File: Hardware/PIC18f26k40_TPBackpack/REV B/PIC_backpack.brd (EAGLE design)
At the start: 45 x 57.5 mm, 61 parts, among them IC1 PIC18F2480-I/ML, T1 BT138-V, T2 BT138-V, U4 W5500, Y2 CRYSTAL-GROUNDEDSMD-3.2X2.5

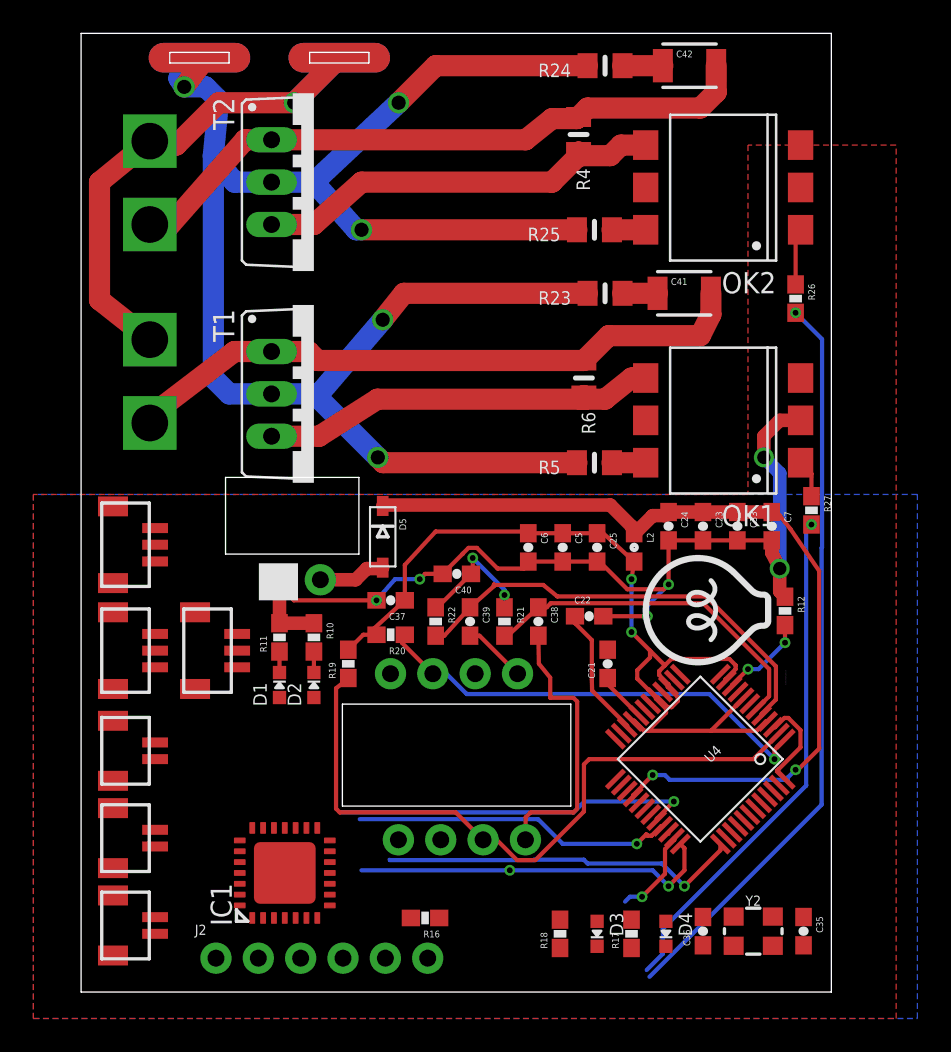
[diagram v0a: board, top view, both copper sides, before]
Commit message: HEEP-414 back to work
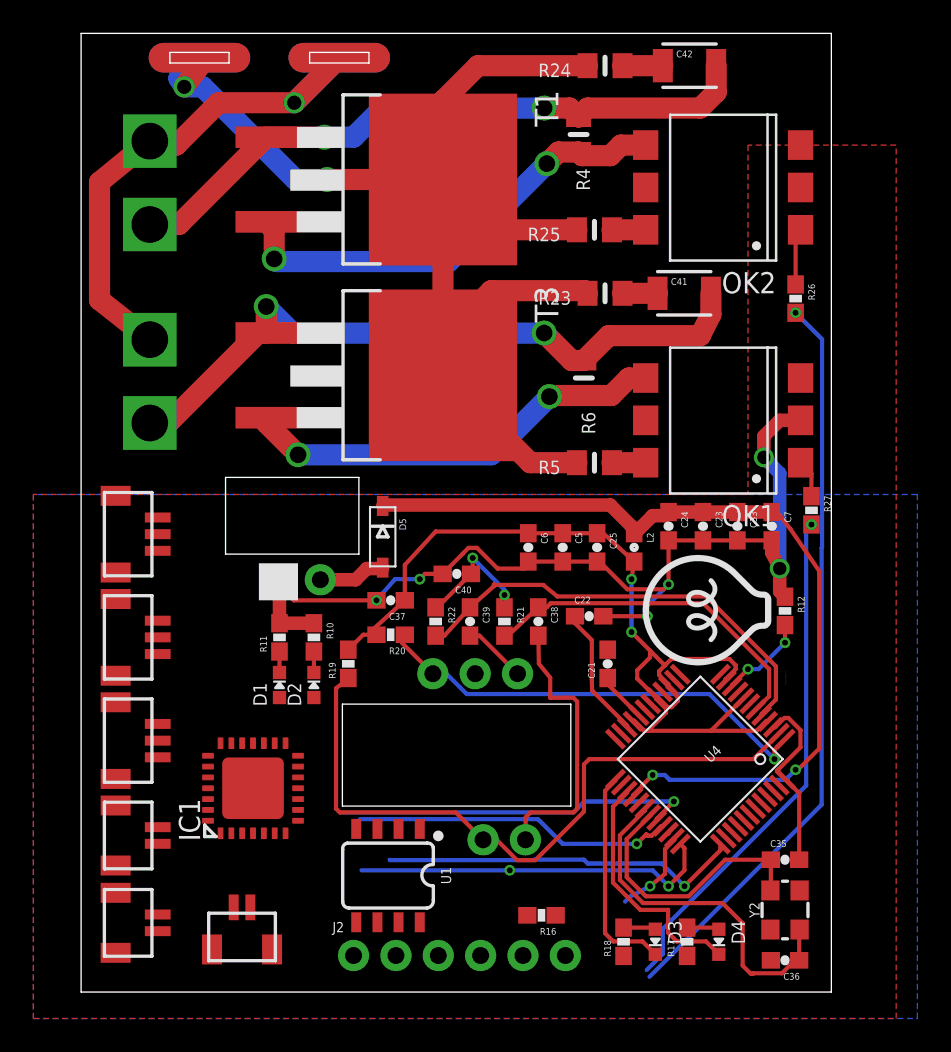
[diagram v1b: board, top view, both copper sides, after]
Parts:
- removed T2: BT138-V, triac:TO220BV
- added T3: BT138, triac:D2PAK-3
- added U1: 4MB Flash, SparkFun-IC-Memory:SO08
- T1: value BT138-V -> BT138; device triac:TO220BV -> triac:D2PAK-3
- U$1: value TPLINK_BACKPACK -> TPLINK_BACKPACKMINIMAL_HOLES; device Heep:BACKPACK_WITH_PROTO -> Heep:BACKPACK_MINIMAL_HOLES
- moved T1 15.7 mm to (11.1, 51.3)
- moved U$14 10.6 mm to (10.2, 5.08), turned to 180 degrees
- moved J2 8.26 mm to (16.4, 2.19)
- moved R16 6.99 mm to (27.6, 4.60)
- moved IC1 5.43 mm to (10.3, 12.2)
- moved U$12 5.40 mm to (4.60, 15.1)
- moved C36 5.22 mm to (42.2, 1.91), turned to 180 degrees
- moved U$13 4.83 mm to (4.60, 21.3)
- moved C35 4.43 mm to (42.2, 7.94), turned to 0 degrees
- moved R18 3.84 mm to (32.5, 3.02)
- moved D3 3.52 mm to (34.4, 3.02)
- moved R17 3.37 mm to (36.4, 3.02)
- moved D4 3.21 mm to (38.3, 3.02)
- moved Y2 2.29 mm to (42.2, 4.92), turned to 90 degrees
- moved U$11 0.65 mm to (4.60, 27.5)
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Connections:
- net GATE: now also T3.G; no longer T1.G
- net GATE2: now also T1.G; no longer T2.G
- net GND: now also U1.4
- net HOT: now also T1.A2, T3.A2; no longer T1.T2, T2.T2
- net LOAD1: now also T3.A1; no longer T1.T1
- net LOAD2: now also T1.A1; no longer T2.T1
- net MISO: now also U1.2
- net MOSI: now also U1.5
- net SCK: now also U1.6
- net VCC: now also U1.8
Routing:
- net HOT: track 109.5 -> 79.8 mm, vias 5 -> 2
- net N$24: track 0.00 -> 21.6 mm
- net N$23: track 0.00 -> 16.3 mm
- net ACTLED: track 0.00 -> 14.8 mm
- net LNKLED: track 0.00 -> 13.0 mm
- net GND: track 69.2 -> 74.4 mm
- net LOAD1: track 37.4 -> 41.5 mm, vias 0 -> 2
- net GATE2: track 24.6 -> 27.8 mm, vias 0 -> 2
- net GATE: track 23.8 -> 25.8 mm, vias 0 -> 2
- net N$12: track 0.00 -> 1.95 mm
- net N$13: track 0.00 -> 1.95 mm
- net LOAD2: track 39.1 -> 39.3 mm, vias 0 -> 2
